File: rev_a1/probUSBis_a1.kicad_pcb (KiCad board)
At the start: 2 copper layers, 44.5 x 22.9 mm, 23 parts, among them CON1 USB-MINI-B, IC1 ATTINY85-P, P1 USB_A_MALE, P2 CONN_8, P3 CONN_4, U1 LM78L05ACZ

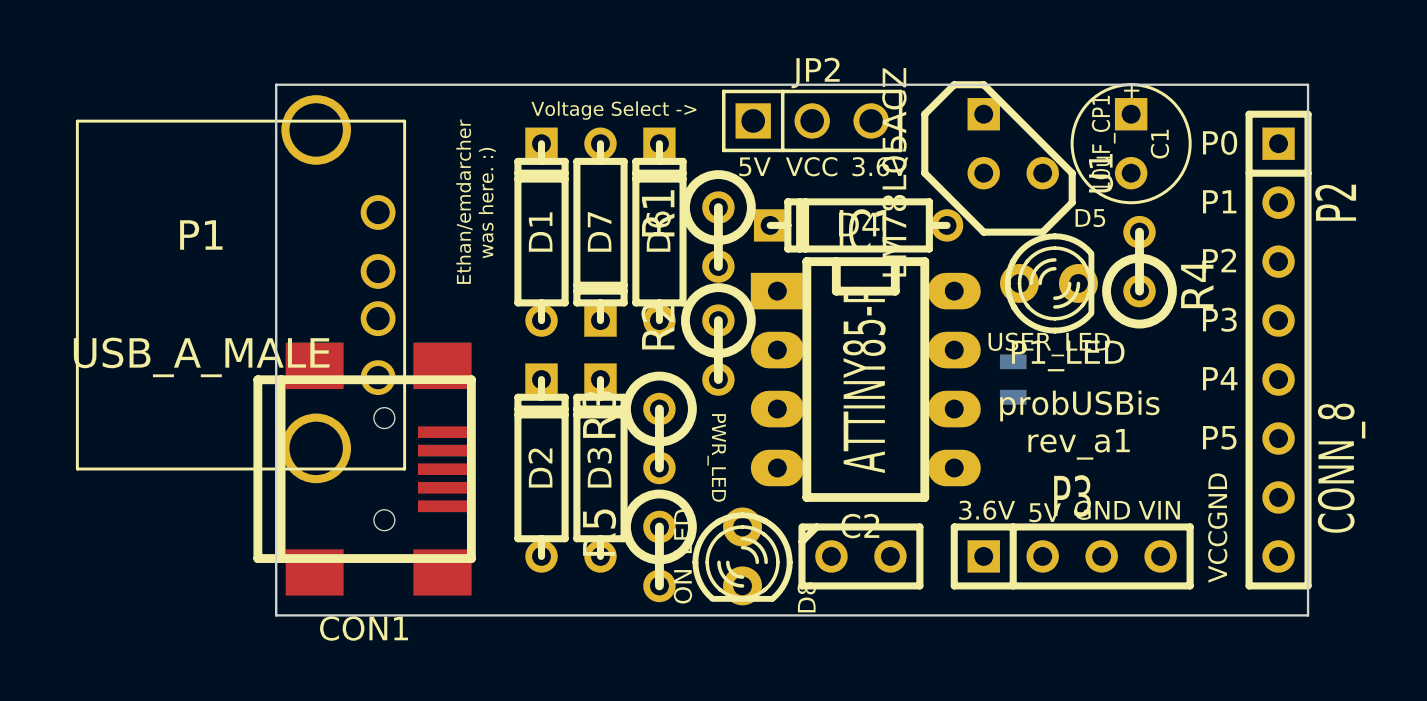
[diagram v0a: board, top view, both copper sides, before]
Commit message: did some routing with freerouter
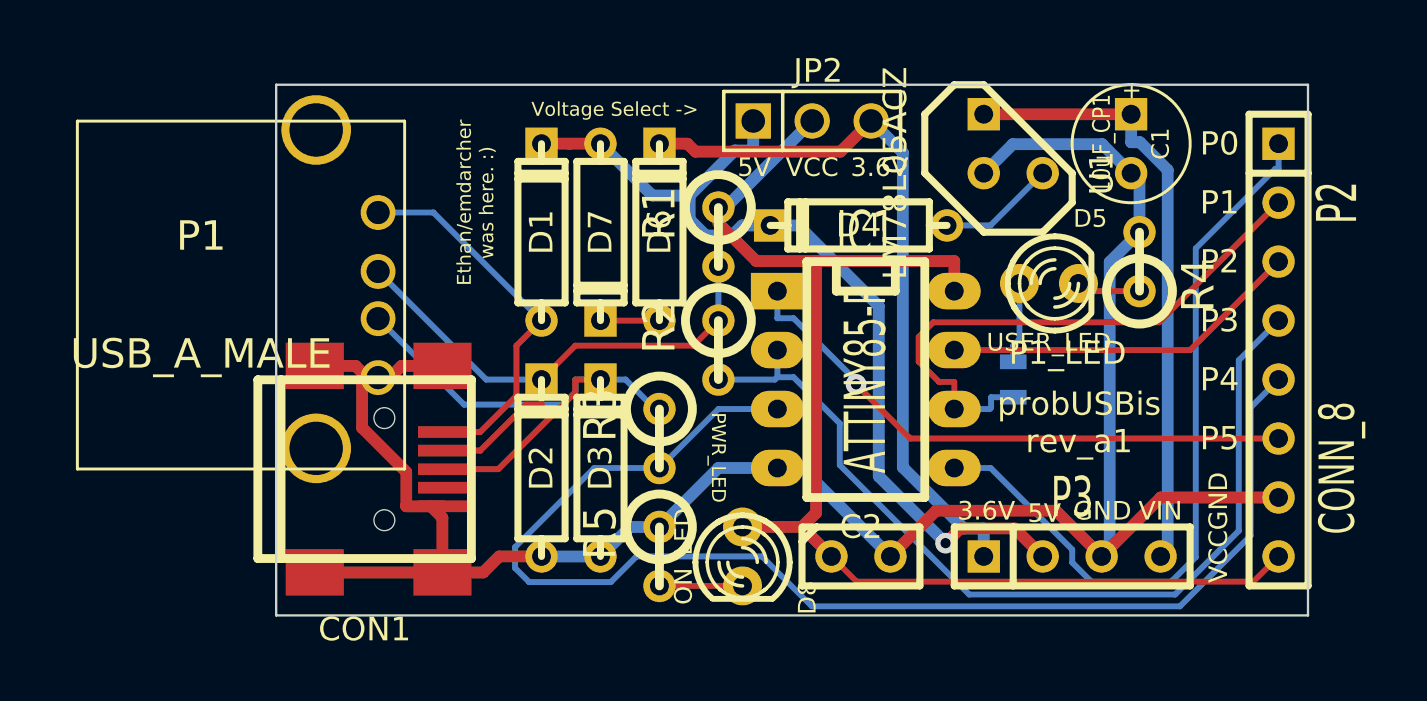
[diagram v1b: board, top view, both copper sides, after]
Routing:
- net GND: track 0.00 -> 90.3 mm
- net N-0000015: track 0.00 -> 56.4 mm
- net VCC: track 0.00 -> 54.6 mm
- net +5V: track 0.00 -> 39.6 mm, vias 0 -> 1
- net N-0000020: track 0.00 -> 39.5 mm
- net N-000006: track 0.00 -> 32.6 mm
- net +3.3V: track 0.00 -> 31.1 mm
- net VIN: track 0.00 -> 26.4 mm
- net N-0000019: track 0.00 -> 26.0 mm
- net N-000007: track 0.00 -> 25.0 mm
- net N-000002: track 0.00 -> 25.0 mm, vias 0 -> 1
- net N-0000017: track 0.00 -> 23.6 mm
- net N-000005: track 0.00 -> 16.4 mm
- net N-000008: track 0.00 -> 15.5 mm
- net N-0000016: track 0.00 -> 5.05 mm
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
